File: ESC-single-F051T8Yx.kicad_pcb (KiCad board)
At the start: 4 copper layers, 15 x 15 mm, 58 parts, among them U1 STM32F051T8Yx, U2 TPS727xxDSE, U3 SIZF360DT-T1-GE3, U4 NCP81253MNTBG, U5 SIZF360DT-T1-GE3, U6 NCP81253MNTBG, U7 SIZF360DT-T1-GE3, U8 NCP81253MNTBG

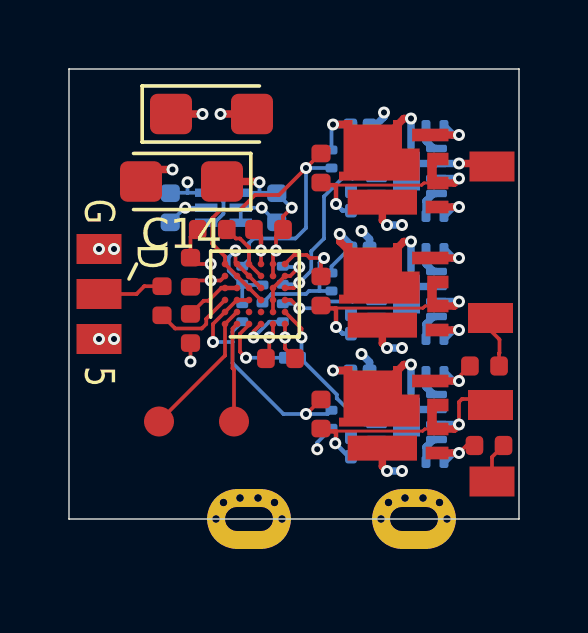
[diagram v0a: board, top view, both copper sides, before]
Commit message: overall update
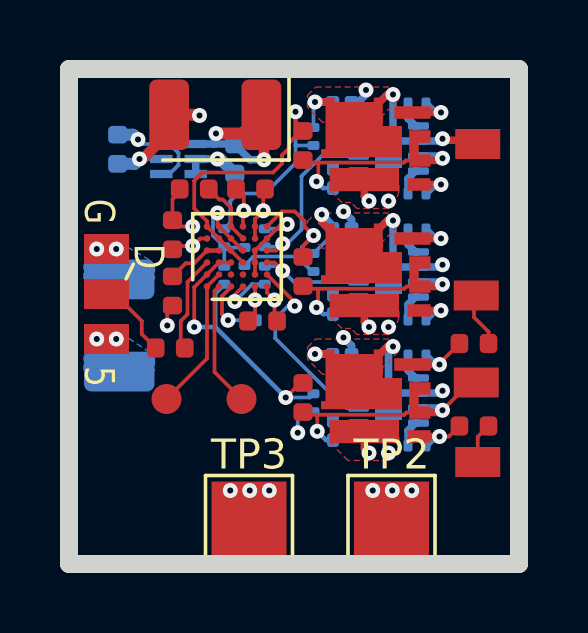
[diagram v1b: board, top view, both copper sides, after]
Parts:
- C13: footprint Capacitor_Tantalum_SMD:CP_EIA-3216-18_Kemet-A -> Capacitor_Tantalum_SMD:CP_EIA-3528-12_Kemet-T; moved to B.Cu
- C14: footprint Capacitor_Tantalum_SMD:CP_EIA-3216-18_Kemet-A -> Capacitor_Tantalum_SMD:CP_EIA-3528-12_Kemet-T
- TP2, TP3: footprint footprints:batt_pad_wide_relaxed -> TestPoint:TestPoint_Pad_2.5x2.5mm
- U3, U5, U7: footprint footprints:PowerPair_3.3x3.3F_BWL -> footprints:PowerPair_3.3x3.3F_BWL_mod
- moved C13 7.69 mm to (51.7, 58.5), turned to 90 degrees
- moved C12 2.62 mm to (51.6, 52.7)
- moved C14 2.49 mm to (54.9, 51.5)
- moved U2 2.21 mm to (53.6, 53.0)
- moved C11 2.14 mm to (55.5, 53.0)
- moved R23 1.60 mm to (53.4, 59.3), turned to 180 degrees
- moved R21 1.53 mm to (56.6, 58.4)
- moved C2 1.48 mm to (56.0, 54.0)
- moved C4 1.48 mm to (54.2, 54.0)
- moved R13 1.39 mm to (55.9, 56.2)
- moved R14 1.39 mm to (56.5, 56.9)
- moved R20 1.39 mm to (55.2, 56.9)
- moved R3 1.39 mm to (55.2, 55.6)
- moved R8 1.39 mm to (56.5, 55.6)
- moved U1 1.39 mm to (55.6, 56.2)
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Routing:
- net GND: track 36.0 -> 40.4 mm, vias 18 -> 22
- net 3V3_route: track 8.65 -> 10.6 mm
- net +BATT: track 3.98 -> 2.33 mm, vias 6 -> 9
- net CL: track 5.28 -> 6.65 mm
- net COM1_INM_C: track 9.05 -> 10.2 mm
- net COM1_INM_A: track 13.7 -> 14.7 mm
- net COM1_INM_B: track 5.67 -> 6.57 mm
- net SWDIO: track 3.33 -> 4.18 mm
- net AH: track 2.53 -> 3.05 mm
- net +5V: track 13.1 -> 13.2 mm, vias 7 -> 6
- added copper zone on B.Cu, net +5V
- added copper zone on F.Cu, net +BATT
- added copper zone on B.Cu, net GND
- added copper zone on F.Cu, net GND
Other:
- board size 15 x 15 mm -> 15 x 16.5 mm
- net class Default: trace_width 0.25 -> 0.125; via_dia 0.8 -> 0.5; via_drill 0.4 -> 0.2
- rule via_min_size: 0.4 -> 0.45
- board text added: "hilariESC v0.1"
- board text removed: "hilariESC v0.1 crteensy"
